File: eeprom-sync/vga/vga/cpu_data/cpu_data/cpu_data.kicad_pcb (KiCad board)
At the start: 2 copper layers, 78.7 x 42.7 mm, 32 parts, among them J1 Conn_02x06_Odd_Even, J10 Conn_01x03_Female, J11 Conn_01x02_Female, J12 Conn_02x05_Odd_Even, J2 Conn_01x02_Female, J3 Conn_01x04_Female, J4 Conn_01x15_Female, J5 Conn_01x15_Female, J6 Conn_02x08_Odd_Even, J7 Conn_01x02_Female, J8 Conn_01x02_Female, J9 Conn_01x08_Female, U1 GAL22V10, U2 74HC14, U3 74LS02, U4 IDT7205L12JG, U5 74LS573

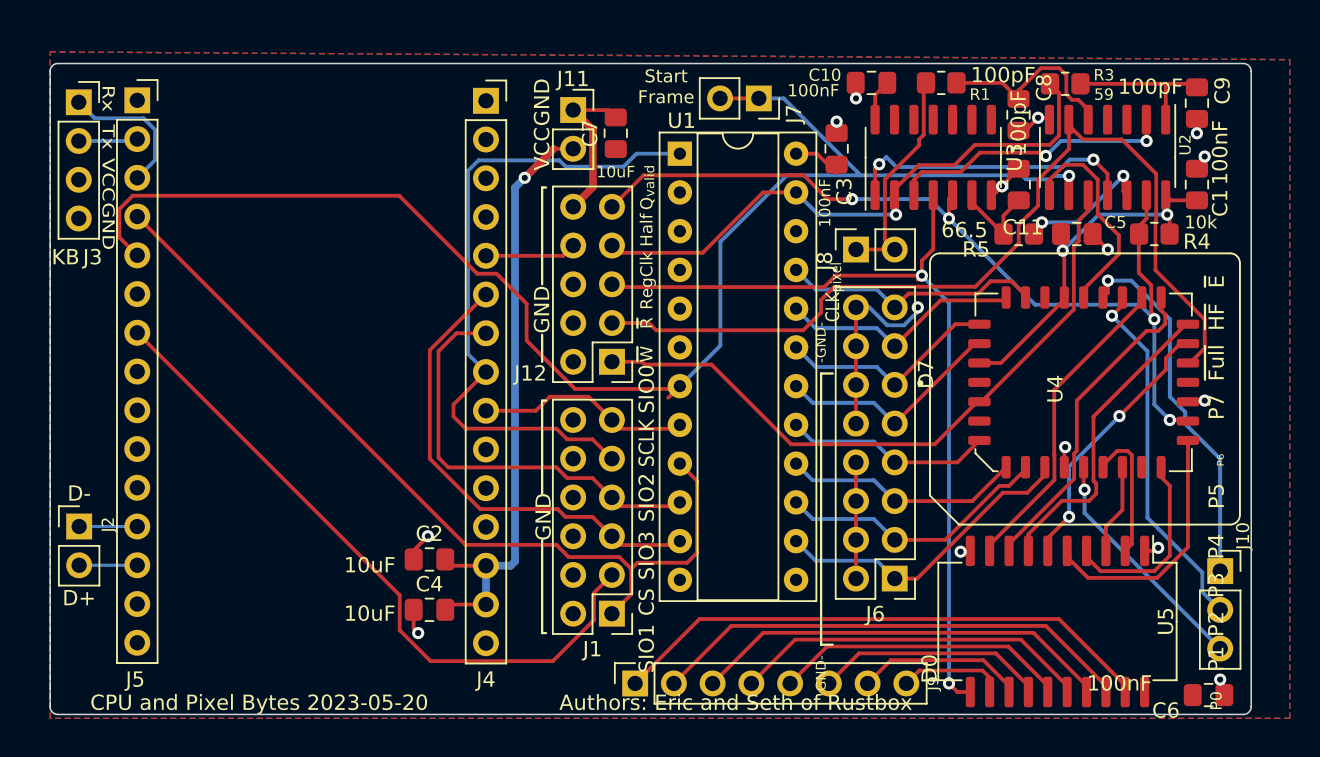
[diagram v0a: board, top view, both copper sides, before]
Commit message: routing completed
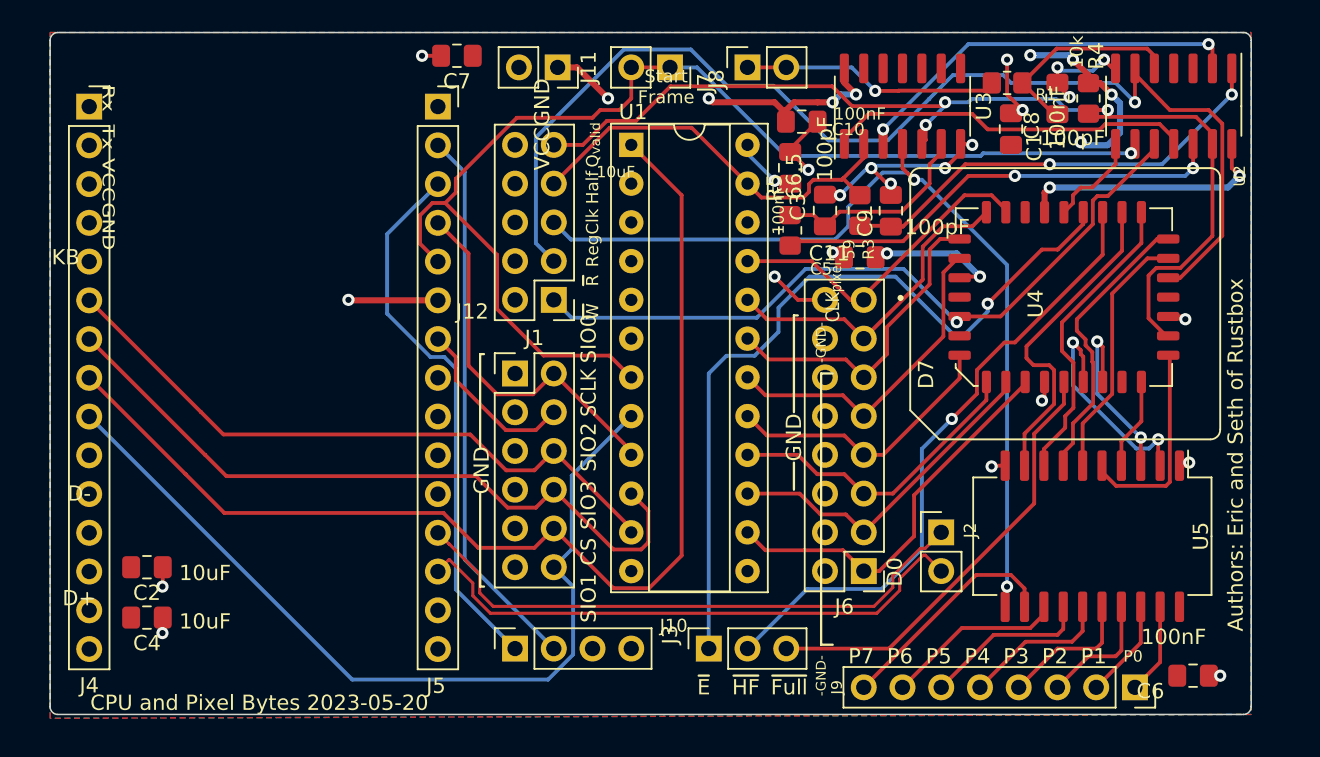
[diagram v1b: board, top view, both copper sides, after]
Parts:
- moved J2 56.5 mm to (134.6, 91.4)
- moved J3 45.8 mm to (106.7, 99.1), turned to 90 degrees
- moved J10 33.9 mm to (119.4, 99.1), turned to 90 degrees
- moved J9 32.8 mm to (147.3, 101.6), turned to -90 degrees
- moved J4 26.0 mm to (78.8, 63.5)
- moved C9 21.3 mm to (131.3, 70.4), turned to 90 degrees
- moved J5 19.7 mm to (101.6, 63.5)
- moved C2 18.5 mm to (82.5, 93.7), turned to 180 degrees
- moved C4 18.5 mm to (82.5, 97.0), turned to 180 degrees
- moved J1 17.0 mm to (106.7, 81.0), turned to 0 degrees
- moved R3 15.8 mm to (129.3, 70.3), turned to -90 degrees
- moved R5 15.0 mm to (124.7, 71.6), turned to -90 degrees
- moved C5 14.3 mm to (129.3, 73.4), turned to 0 degrees
- moved J8 13.9 mm to (121.9, 61.0)
- moved C11 12.8 mm to (127.0, 70.3)
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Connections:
- J1 pad 1: /SIO1 -> GND
- J1 pad 10: GND -> /SCLK
- J1 pad 11: /SIO0 -> GND
- J1 pad 12: GND -> /SIO0
- J1 pad 2: GND -> /SIO1
- J1 pad 3: /CS -> GND
- J1 pad 4: GND -> /CS
- J1 pad 5: /SIO3 -> GND
- J1 pad 6: GND -> /SIO3
- J1 pad 7: /SIO2 -> GND
- J1 pad 8: GND -> /SIO2
- J1 pad 9: /SCLK -> GND
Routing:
- net /SIO0: track 13.8 -> 57.8 mm
- net /D-: track 3.81 -> 38.2 mm
- net /D+: track 3.81 -> 37.8 mm
- net /CS: track 44.8 -> 11.4 mm
- net /KB_{Tx}: track 3.89 -> 36.1 mm
- net /SIO1: track 56.5 -> 24.6 mm
- net /SCLK: track 44.1 -> 74.8 mm
- net /P0: track 36.1 -> 5.96 mm
- net /Empty: track 24.2 -> 51.8 mm
- net /KB_{Rx}: track 9.39 -> 35.9 mm
- net /P1: track 31.9 -> 6.49 mm
- net Net-(R5-Pad2): track 8.94 -> 30.1 mm
- net /P2: track 27.7 -> 8.06 mm
- net Net-(C9-Pad1): track 10.1 -> 29.7 mm, vias 0 -> 2
- net /SIO2: track 27.6 -> 47.2 mm
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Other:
- board size 78.7 x 42.7 mm -> 78.7 x 44.7 mm
